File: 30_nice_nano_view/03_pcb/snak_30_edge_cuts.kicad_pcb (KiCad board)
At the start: 2 copper layers, 114 x 99 mm, 118 parts

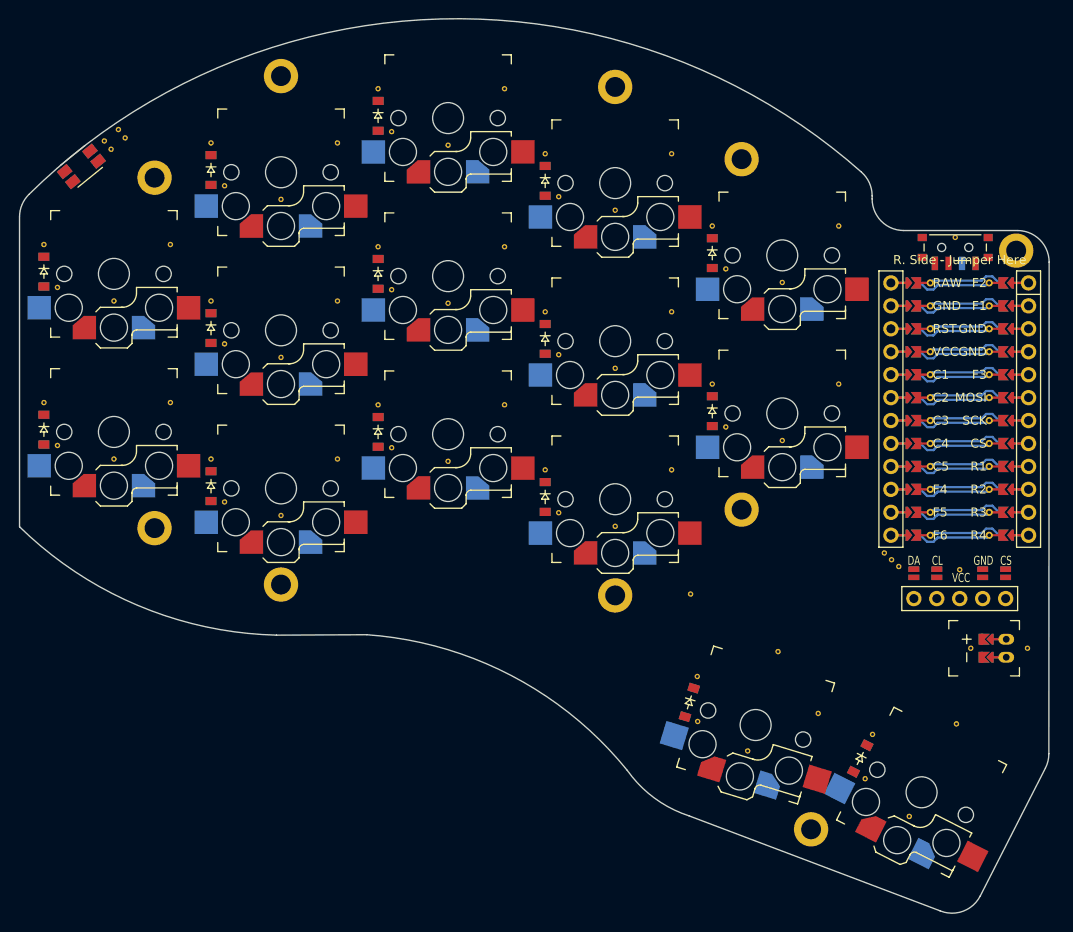
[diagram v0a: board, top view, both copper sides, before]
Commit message: update 30 key nicenano board
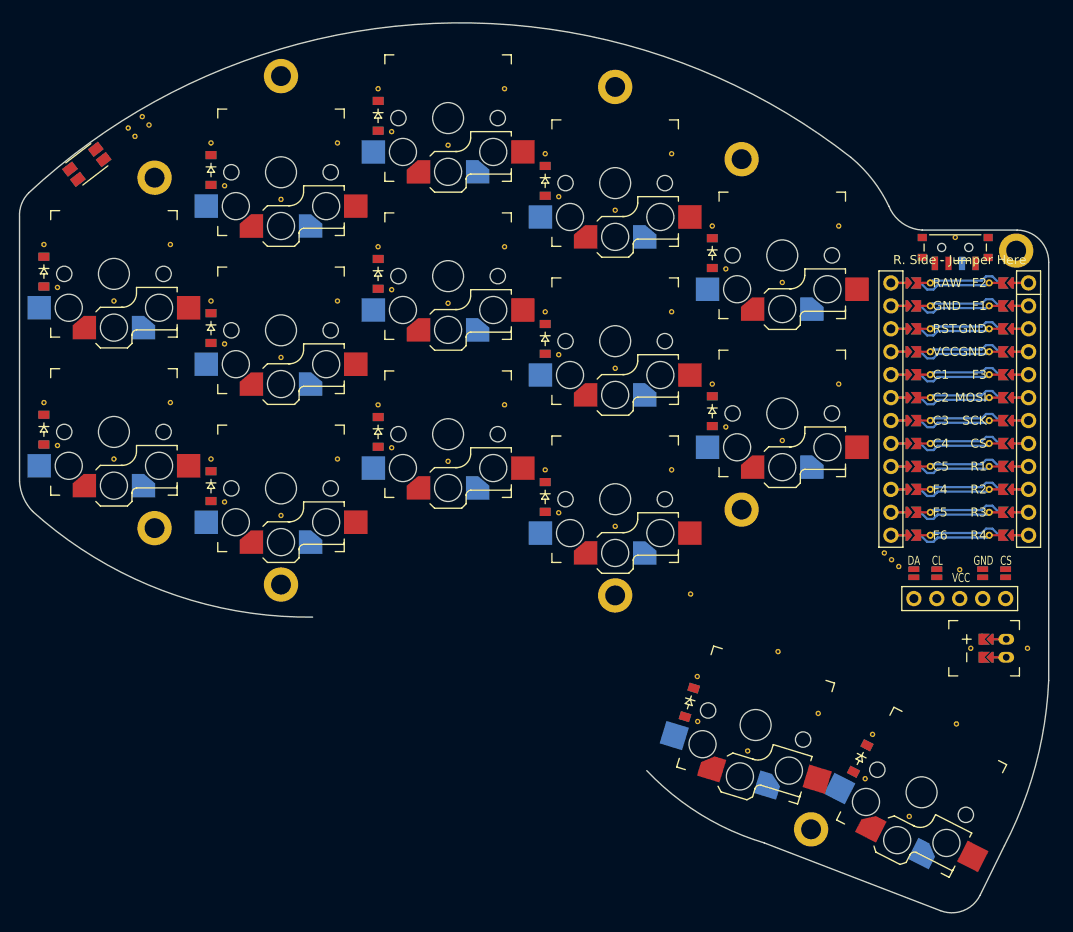
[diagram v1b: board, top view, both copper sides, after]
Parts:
- moved REF** 3.00 mm to (101.6, 48.8)
- moved REF** 3.00 mm to (102.3, 49.8)
- moved REF** 3.00 mm to (103.1, 47.6)
- moved REF** 3.00 mm to (103.9, 48.5)
- moved SW2 0.64 mm to (97.0, 52.9), turned to 127.5 degrees
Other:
- board size 114 x 99 mm -> 114 x 98.5 mm
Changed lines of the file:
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@@
   )
   (footprint "VIA-0.6mm" (layer "F.Cu")
-    (at 100.494144 49.019006 129)
+    (at 103.137109 47.589196 129)
     (attr through_hole)
     (fp_text reference "REF**" (at 0 1.4) (layer "F.SilkS") hide
@@
   )
   (footprint "VIA-0.6mm" (layer "F.Cu")
-    (at 101.243035 49.94381 129)
+    (at 103.886 48.514 129)
     (attr through_hole)
     (fp_text reference "REF**" (at 0 1.4) (layer "F.SilkS") hide
@@
   )
   (footprint "VIA-0.6mm" (layer "F.Cu")
-    (at 98.939852 50.277647 129)
+    (at 101.582817 48.847837 129)
     (attr through_hole)
     (fp_text reference "REF**" (at 0 1.4) (layer "F.SilkS") hide
@@
   )
   (footprint "sw_reset_side" (layer "F.Cu")
-    (at 96.4 53.1 129)
+    (at 97 52.87 127.5)
     (attr smd)
-    (fp_text reference "SW2" (at 0 3.5 129) (layer "F.SilkS") hide
+    (fp_text reference "SW2" (at 0 3.5 127.5) (layer "F.SilkS") hide
         (effects (font (size 1 1) (thickness 0.15)))
     )
-    (fp_text value "" (at 0 0 129) (layer "F.SilkS")
+    (fp_text value "" (at 0 0 127.5) (layer "F.SilkS")
         (effects (font (size 1.27 1.27) (thickness 0.15)))
     )
-    (fp_text user "SW2" (at 0 3.5 129) (layer "B.SilkS") hide
+    (fp_text user "SW2" (at 0 3.5 127.5) (layer "B.SilkS") hide
         (effects (font (size 1 1) (thickness 0.15)) (justify mirror))
     )
@@
     (fp_line (start 2.1 0.85) (end 2.1 -0.85)
       (stroke (width 0.1) (type solid)) (layer "F.Fab"))
-    (pad "1" smd rect (at -0.72 -1.8 219) (size 1.4 1.05) (layers "F.Cu" "F.Paste" "F.Mask")
+    (pad "1" smd rect (at -0.72 -1.8 217.5) (size 1.4 1.05) (layers "F.Cu" "F.Paste" "F.Mask")
       (net 26 "GND"))
-    (pad "1" smd rect (at -0.72 -1.8 39) (size 1.4 1.05) (layers "B.Cu" "B.Paste" "B.Mask")
+    (pad "1" smd rect (at -0.72 -1.8 37.5) (size 1.4 1.05) (layers "B.Cu" "B.Paste" "B.Mask")
       (net 26 "GND"))
-    (pad "1" smd rect (at -0.72 1.8 219) (size 1.4 1.05) (layers "F.Cu" "F.Paste" "F.Mask")
+    (pad "1" smd rect (at -0.72 1.8 217.5) (size 1.4 1.05) (layers "F.Cu" "F.Paste" "F.Mask")
       (net 26 "GND"))
-    (pad "1" smd rect (at -0.72 1.8 39) (size 1.4 1.05) (layers "B.Cu" "B.Paste" "B.Mask")
+    (pad "1" smd rect (at -0.72 1.8 37.5) (size 1.4 1.05) (layers "B.Cu" "B.Paste" "B.Mask")
       (net 26 "GND"))
-    (pad "2" smd rect (at 0.72 -1.8 219) (size 1.4 1.05) (layers "F.Cu" "F.Paste" "F.Mask")
+    (pad "2" smd rect (at 0.72 -1.8 217.5) (size 1.4 1.05) (layers "F.Cu" "F.Paste" "F.Mask")
       (net 27 "RST"))
-    (pad "2" smd rect (at 0.72 -1.8 39) (size 1.4 1.05) (layers "B.Cu" "B.Paste" "B.Mask")
+    (pad "2" smd rect (at 0.72 -1.8 37.5) (size 1.4 1.05) (layers "B.Cu" "B.Paste" "B.Mask")
       (net 27 "RST"))
-    (pad "2" smd rect (at 0.72 1.8 219) (size 1.4 1.05) (layers "F.Cu" "F.Paste" "F.Mask")
+    (pad "2" smd rect (at 0.72 1.8 217.5) (size 1.4 1.05) (layers "F.Cu" "F.Paste" "F.Mask")
       (net 27 "RST"))
-    (pad "2" smd rect (at 0.72 1.8 39) (size 1.4 1.05) (layers "B.Cu" "B.Paste" "B.Mask")
+    (pad "2" smd rect (at 0.72 1.8 37.5) (size 1.4 1.05) (layers "B.Cu" "B.Paste" "B.Mask")
       (net 27 "RST"))
   )
@@
   )
   (footprint "VIA-0.6mm" (layer "F.Cu")
-    (at 99.688743 51.20245 129)
+    (at 102.331708 49.77264 129)
     (attr through_hole)
     (fp_text reference "REF**" (at 0 1.4) (layer "F.SilkS") hide
@@
   (gr_circle (center 118.5 99.4) (end 120 99.4)
     (stroke (width 0.15) (type solid)) (fill none) (layer "Eco2.User"))
-  (gr_line (start 203.13565 119.719514) (end 195.923145 133.874853)
+  (gr_arc (start 172 128) (mid 164.97339 124.855741) (end 159 120)
     (stroke (width 0.15) (type solid)) (layer "Edge.Cuts"))
-  (gr_arc (start 187.45 60.2) (mid 184.975126 59.174874) (end 183.95 56.7)
+  (gr_line (start 198.6 128.3) (end 195.9 133.8)
     (stroke (width 0.15) (type solid)) (layer "Edge.Cuts"))
-  (gr_line (start 89.55 93) (end 89.55 58.692372)
+  (gr_arc (start 189.5 60.15) (mid 187.263797 59.364226) (end 185.8 57.5)
     (stroke (width 0.15) (type solid)) (layer "Edge.Cuts"))
-  (gr_arc (start 163.66 124.999999) (mid 159.844543 123.03625) (end 156.839956 119.972513)
+  (gr_line (start 89.55 88) (end 89.55 58.7)
     (stroke (width 0.15) (type solid)) (layer "Edge.Cuts"))
-  (gr_line (start 187.45 60.2) (end 200.048013 60.2)
+  (gr_line (start 189.5 60.15) (end 200 60.15)
     (stroke (width 0.15) (type solid)) (layer "Edge.Cuts"))
-  (gr_arc (start 89.55 58.692372) (mid 89.820936 57.342133) (end 90.591797 56.200939)
+  (gr_arc (start 89.55 58.7) (mid 89.780852 57.235609) (end 90.6 56)
     (stroke (width 0.15) (type solid)) (layer "Edge.Cuts"))
-  (gr_arc (start 203.517127 118.132533) (mid 203.42019 118.948572) (end 203.13565 119.719514)
+  (gr_arc (start 203.5 110) (mid 202.052088 119.418319) (end 198.6 128.3)
     (stroke (width 0.15) (type solid)) (layer "Edge.Cuts"))
-  (gr_line (start 183.95 56.7) (end 183.95 56.354306)
+  (gr_line (start 203.5 63.7) (end 203.5 110)
     (stroke (width 0.15) (type solid)) (layer "Edge.Cuts"))
-  (gr_line (start 203.548013 63.701986) (end 203.517127 118.132533)
+  (gr_arc (start 91 91.3) (mid 89.98406 89.777837) (end 89.55 88)
     (stroke (width 0.15) (type solid)) (layer "Edge.Cuts"))
-  (gr_arc (start 195.923145 133.874853) (mid 194.021857 135.567401) (end 191.476715 135.524198)
+  (gr_arc (start 195.9 133.8) (mid 194.031815 135.508815) (end 191.5 135.5)
     (stroke (width 0.15) (type solid)) (layer "Edge.Cuts"))
-  (gr_arc (start 200.048013 60.199999) (mid 202.523589 61.225828) (end 203.548013 63.701986)
+  (gr_arc (start 200 60.15) (mid 202.485523 61.199837) (end 203.5 63.7)
     (stroke (width 0.15) (type solid)) (layer "Edge.Cuts"))
-  (gr_arc (start 118 105) (mid 102.635557 101.701429) (end 89.55 93)
+  (gr_arc (start 181.6 52.1) (mid 183.995505 54.570163) (end 185.8 57.5)
     (stroke (width 0.15) (type solid)) (layer "Edge.Cuts"))
-  (gr_arc (start 182.771484 53.73501) (mid 183.641801 54.918199) (end 183.95 56.354306)
+  (gr_arc (start 90.6 56) (mid 135.380905 37.271116) (end 181.6 52.1)
     (stroke (width 0.15) (type solid)) (layer "Edge.Cuts"))
-  (gr_line (start 128.003322 104.952626) (end 118 105)
+  (gr_line (start 191.5 135.5) (end 172 128)
     (stroke (width 0.15) (type solid)) (layer "Edge.Cuts"))
-  (gr_arc (start 90.591797 56.200939) (mid 136.194931 36.77414) (end 182.771484 53.73501)
-    (stroke (width 0.15) (type solid)) (layer "Edge.Cuts"))
-  (gr_line (start 191.476715 135.524198) (end 163.66 125)
-    (stroke (width 0.15) (type solid)) (layer "Edge.Cuts"))
-  (gr_arc (start 128.003322 104.952626) (mid 143.983857 109.463271) (end 156.839955 119.972514)
+  (gr_arc (start 122 103) (mid 105.398912 100.067413) (end 91 91.3)
     (stroke (width 0.15) (type solid)) (layer "Edge.Cuts"))
+  (gr_arc (start 122 103) (mid 142.325339 107.527204) (end 159 120)
+    (stroke (width 0.15) (type solid)) (layer "F.Fab"))
   (segment (start 198.43 76.16) (end 196.91 76.16) (width 0.25) (layer "F.Cu") (net 1))
   (segment (start 191.11 76.51) (end 191.11 76.5) (width 0.25) (layer "B.Cu") (net 1))

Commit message: update
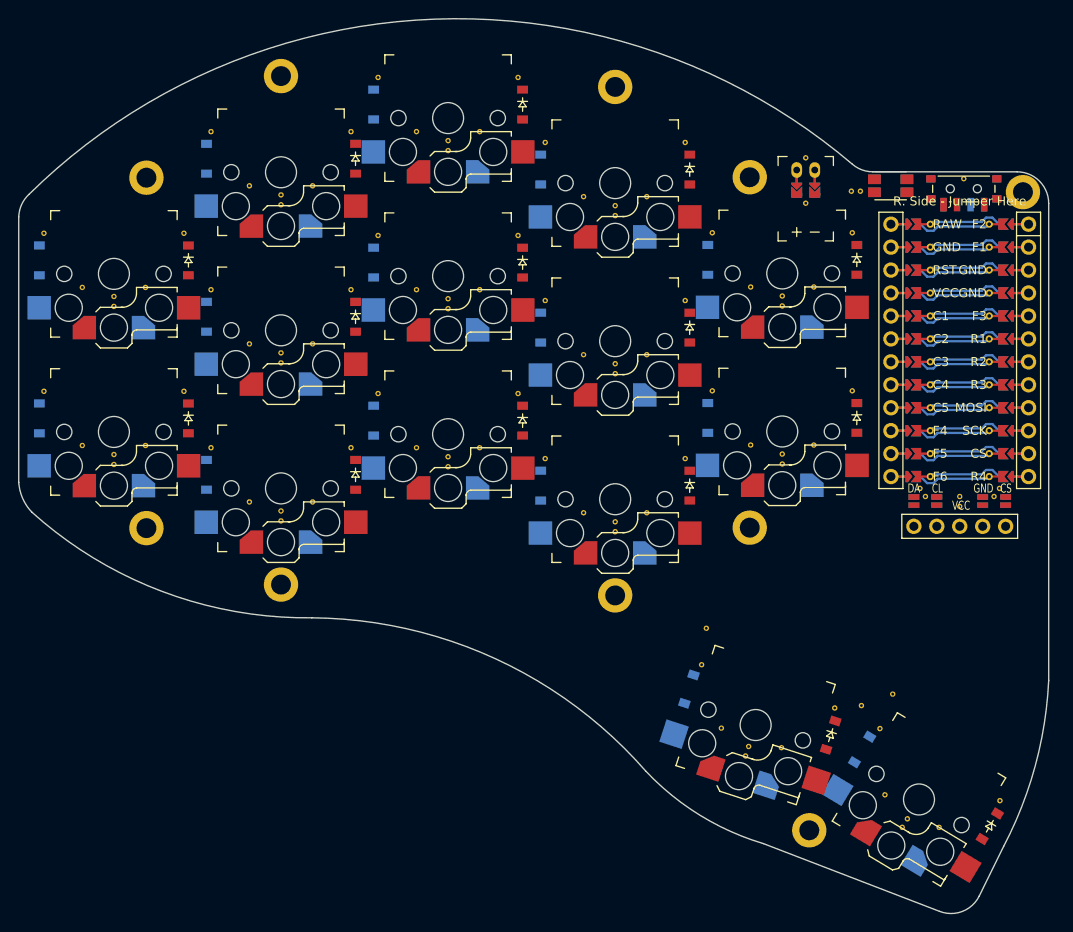
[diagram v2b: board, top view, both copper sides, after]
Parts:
- removed the REF** at (193.2, 61.0)
- removed the REF** at (161.8, 86.7)
- removed the REF** at (137.0, 85.8)
- removed the REF** at (103.1, 47.6)
- removed the REF** at (106.2, 61.8)
- removed the REF** at (106.2, 79.2)
- removed the REF** at (143.2, 79.5)
- removed the REF** at (149.2, 74.0)
- removed the REF** at (186.1, 96.7)
- removed the REF** at (118.5, 91.8)
- removed the REF** at (124.8, 50.5)
- removed the REF** at (155.5, 93.0)
- removed the REF** at (92.2, 79.2)
- removed the REF** at (184.0, 116.0)
- removed the REF** at (149.2, 56.5)
- removed the REF** at (103.9, 48.5)
- removed the REF** at (110.8, 68.0)
- removed the REF** at (174.0, 83.5)
- removed the REF** at (101.6, 48.8)
- removed the REF** at (161.8, 69.2)
- removed the REF** at (130.8, 49.2)
- removed the REF** at (100.0, 68.0)
- removed the REF** at (124.8, 85.5)
- removed the REF** at (112.2, 90.2)
- removed the REF** at (166.2, 59.7)
- removed the REF** at (118.5, 74.2)
- removed the REF** at (110.8, 85.5)
- removed the REF** at (170.2, 117.8)
- removed the REF** at (186.9, 97.4)
- removed the REF** at (155.5, 75.5)
- removed the REF** at (155.5, 58.0)
- removed the REF** at (137.0, 68.2)
- removed the REF** at (178.0, 113.7)
- removed the REF** at (124.8, 68.0)
- removed the REF** at (167.8, 64.5)
- removed the REF** at (173.5, 106.8)
- removed the REF** at (149.2, 91.5)
- removed the REF** at (130.8, 66.8)
- removed the REF** at (167.8, 82.0)
- removed the REF** at (147.8, 86.7)
- removed the REF** at (166.2, 77.2)
- removed the REF** at (164.6, 114.6)
- removed the REF** at (194.9, 106.5)
- removed the REF** at (129.2, 44.5)
- removed the REF** at (174.0, 66.0)
- removed the REF** at (118.5, 56.8)
- removed the REF** at (163.8, 100.5)
- removed the REF** at (188.1, 125.1)
- removed the REF** at (92.2, 61.8)
- removed the REF** at (183.2, 120.9)
- removed the REF** at (201.2, 106.5)
- removed the REF** at (143.2, 62.0)
- removed the REF** at (185.3, 95.9)
- removed the REF** at (147.8, 69.2)
- removed the REF** at (143.2, 44.5)
- removed the REF** at (193.3, 114.8)
- removed the REF** at (193.7, 97.8)
- removed the REF** at (110.8, 50.5)
- removed the REF** at (93.8, 84.0)
- removed the REF** at (130.8, 84.2)
- removed the REF** at (164.6, 109.6)
- removed the REF** at (137.0, 50.8)
- removed the REF** at (102.3, 49.8)
- removed the REF** at (100.0, 85.5)
- removed the REF** at (112.2, 72.8)
- removed the REF** at (180.2, 59.7)
- removed the REF** at (147.8, 51.7)
- removed the REF** at (93.8, 66.5)
- removed the REF** at (180.2, 77.2)
- removed the REF** at (129.2, 79.5)
- removed the REF** at (161.8, 51.7)
- removed the REF** at (129.2, 62.0)
- removed the REF** at (112.2, 55.2)
- added D16: , ceoloide:diode_tht_sod123, B.Cu at (91.8, 81.0)
- added D17: , ceoloide:diode_tht_sod123, B.Cu at (91.8, 63.5)
- added D18: , ceoloide:diode_tht_sod123, B.Cu at (110.2, 87.2)
- added D19: , ceoloide:diode_tht_sod123, B.Cu at (110.2, 69.8)
- added D20: , ceoloide:diode_tht_sod123, B.Cu at (110.2, 52.2)
- added D21: , ceoloide:diode_tht_sod123, B.Cu at (128.8, 81.2)
- added D22: , ceoloide:diode_tht_sod123, B.Cu at (128.8, 63.8)
- added D23: , ceoloide:diode_tht_sod123, B.Cu at (128.8, 46.2)
- added D24: , ceoloide:diode_tht_sod123, B.Cu at (147.2, 88.5)
- added D25: , ceoloide:diode_tht_sod123, B.Cu at (147.2, 71.0)
- added D26: , ceoloide:diode_tht_sod123, B.Cu at (147.2, 53.5)
- added D27: , ceoloide:diode_tht_sod123, B.Cu at (165.8, 81.0)
- added D28: , ceoloide:diode_tht_sod123, B.Cu at (165.8, 63.5)
- added D29: , ceoloide:diode_tht_sod123, B.Cu at (163.7, 111.0)
- added D30: , ceoloide:diode_tht_sod123, B.Cu at (182.8, 117.7)
- added REF**: VIA-0.6mm, VIA-0.6mm, F.Cu at (152.0, 56.5)
- added REF**: VIA-0.6mm, VIA-0.6mm, F.Cu at (107.8, 60.5)
- added REF**: VIA-0.6mm, VIA-0.6mm, F.Cu at (155.5, 57.5)
- added REF**: VIA-0.6mm, VIA-0.6mm, F.Cu at (163.2, 85.5)
- added REF**: VIA-0.6mm, VIA-0.6mm, F.Cu at (189.2, 88.8)
- added REF**: VIA-0.6mm, VIA-0.6mm, F.Cu at (122.0, 90.2)
- added REF**: VIA-0.6mm, VIA-0.6mm, F.Cu at (155.5, 92.5)
- added REF**: VIA-0.6mm, VIA-0.6mm, F.Cu at (122.0, 72.8)
- added REF**: VIA-0.6mm, VIA-0.6mm, F.Cu at (197.4, 89.7)
- added REF**: VIA-0.6mm, VIA-0.6mm, F.Cu at (144.8, 60.8)
- added REF**: VIA-0.6mm, VIA-0.6mm, F.Cu at (118.5, 73.8)
- added REF**: VIA-0.6mm, VIA-0.6mm, F.Cu at (96.5, 66.5)
- added REF**: VIA-0.6mm, VIA-0.6mm, F.Cu at (155.5, 58.5)
- added REF**: VIA-0.6mm, VIA-0.6mm, F.Cu at (118.5, 74.8)
- added REF**: VIA-0.6mm, VIA-0.6mm, F.Cu at (181.8, 60.5)
- added REF**: VIA-0.6mm, VIA-0.6mm, F.Cu at (166.2, 78.0)
- added REF**: VIA-0.6mm, VIA-0.6mm, F.Cu at (182.7, 55.8)
- added REF**: VIA-0.6mm, VIA-0.6mm, F.Cu at (167.3, 115.3)
- added REF**: VIA-0.6mm, VIA-0.6mm, F.Cu at (133.5, 66.8)
- added REF**: VIA-0.6mm, VIA-0.6mm, F.Cu at (159.0, 74.0)
- added REF**: VIA-0.6mm, VIA-0.6mm, F.Cu at (182.8, 112.8)
- added REF**: VIA-0.6mm, VIA-0.6mm, F.Cu at (137.0, 85.2)
- added REF**: VIA-0.6mm, VIA-0.6mm, F.Cu at (107.8, 78.0)
- added REF**: VIA-0.6mm, VIA-0.6mm, F.Cu at (144.8, 78.2)
- added REF**: VIA-0.6mm, VIA-0.6mm, F.Cu at (133.5, 49.2)
- added REF**: VIA-0.6mm, VIA-0.6mm, F.Cu at (179.8, 113.1)
- added REF**: VIA-0.6mm, VIA-0.6mm, F.Cu at (173.9, 117.5)
- added REF**: VIA-0.6mm, VIA-0.6mm, F.Cu at (110.8, 84.2)
- added REF**: VIA-0.6mm, VIA-0.6mm, F.Cu at (144.8, 43.2)
- added REF**: VIA-0.6mm, VIA-0.6mm, F.Cu at (103.5, 66.5)
- added REF**: VIA-0.6mm, VIA-0.6mm, F.Cu at (118.5, 91.2)
- added REF**: VIA-0.6mm, VIA-0.6mm, F.Cu at (122.0, 55.2)
- added REF**: VIA-0.6mm, VIA-0.6mm, F.Cu at (100.0, 67.5)
- added REF**: VIA-0.6mm, VIA-0.6mm, F.Cu at (163.2, 50.5)
- added REF**: VIA-0.6mm, VIA-0.6mm, F.Cu at (110.8, 66.8)
- added REF**: VIA-0.6mm, VIA-0.6mm, F.Cu at (137.0, 86.3)
- added REF**: VIA-0.6mm, VIA-0.6mm, F.Cu at (184.8, 115.3)
- added REF**: VIA-0.6mm, VIA-0.6mm, F.Cu at (129.2, 60.8)
- added REF**: VIA-0.6mm, VIA-0.6mm, F.Cu at (140.5, 84.2)
- added REF**: VIA-0.6mm, VIA-0.6mm, F.Cu at (126.2, 49.2)
- added REF**: VIA-0.6mm, VIA-0.6mm, F.Cu at (140.5, 49.2)
- added REF**: VIA-0.6mm, VIA-0.6mm, F.Cu at (126.2, 84.2)
- added REF**: VIA-0.6mm, VIA-0.6mm, F.Cu at (129.2, 43.2)
- added REF**: VIA-0.6mm, VIA-0.6mm, F.Cu at (110.8, 49.2)
- added REF**: VIA-0.6mm, VIA-0.6mm, F.Cu at (100.0, 85.0)
- added REF**: VIA-0.6mm, VIA-0.6mm, F.Cu at (155.5, 76.0)
- added REF**: VIA-0.6mm, VIA-0.6mm, F.Cu at (140.5, 66.8)
- added REF**: VIA-0.6mm, VIA-0.6mm, F.Cu at (115.0, 72.8)
- added REF**: VIA-0.6mm, VIA-0.6mm, F.Cu at (165.6, 104.2)
- added REF**: VIA-0.6mm, VIA-0.6mm, F.Cu at (137.0, 67.8)
- added REF**: VIA-0.6mm, VIA-0.6mm, F.Cu at (189.8, 89.7)
- added REF**: VIA-0.6mm, VIA-0.6mm, F.Cu at (152.0, 91.5)
- added REF**: VIA-0.6mm, VIA-0.6mm, F.Cu at (103.5, 84.0)
- added REF**: VIA-0.6mm, VIA-0.6mm, F.Cu at (155.5, 75.0)
- added REF**: VIA-0.6mm, VIA-0.6mm, F.Cu at (118.5, 56.2)
- added REF**: VIA-0.6mm, VIA-0.6mm, F.Cu at (118.5, 57.4)
- added REF**: VIA-0.6mm, VIA-0.6mm, F.Cu at (181.7, 55.8)
- added REF**: VIA-0.6mm, VIA-0.6mm, F.Cu at (198.1, 88.8)
- added REF**: VIA-0.6mm, VIA-0.6mm, F.Cu at (185.4, 122.7)
- added REF**: VIA-0.6mm, VIA-0.6mm, F.Cu at (137.0, 50.2)
- added REF**: VIA-0.6mm, VIA-0.6mm, F.Cu at (137.0, 68.8)
- added REF**: VIA-0.6mm, VIA-0.6mm, F.Cu at (159.0, 56.5)
- added REF**: VIA-0.6mm, VIA-0.6mm, F.Cu at (92.2, 78.0)
- added REF**: VIA-0.6mm, VIA-0.6mm, F.Cu at (191.4, 126.3)
- added REF**: VIA-0.6mm, VIA-0.6mm, F.Cu at (193.7, 90.8)
- added REF**: VIA-0.6mm, VIA-0.6mm, F.Cu at (115.0, 90.2)
- added REF**: VIA-0.6mm, VIA-0.6mm, F.Cu at (194.1, 54.5)
- added REF**: VIA-0.6mm, VIA-0.6mm, F.Cu at (193.7, 89.7)
- added REF**: VIA-0.6mm, VIA-0.6mm, F.Cu at (177.5, 84.0)
- added REF**: VIA-0.6mm, VIA-0.6mm, F.Cu at (170.3, 117.3)
- added REF**: VIA-0.6mm, VIA-0.6mm, F.Cu at (137.0, 51.4)
- added REF**: VIA-0.6mm, VIA-0.6mm, F.Cu at (174.0, 67.5)
- added REF**: VIA-0.6mm, VIA-0.6mm, F.Cu at (166.2, 60.5)
- added REF**: VIA-0.6mm, VIA-0.6mm, F.Cu at (176.6, 57.2)
- added REF**: VIA-0.6mm, VIA-0.6mm, F.Cu at (186.2, 111.5)
- added REF**: VIA-0.6mm, VIA-0.6mm, F.Cu at (163.2, 68.0)
- added REF**: VIA-0.6mm, VIA-0.6mm, F.Cu at (147.8, 68.0)
- added REF**: VIA-0.6mm, VIA-0.6mm, F.Cu at (133.5, 84.2)
- added REF**: VIA-0.6mm, VIA-0.6mm, F.Cu at (118.5, 92.3)
- added REF**: VIA-0.6mm, VIA-0.6mm, F.Cu at (159.0, 91.5)
- added REF**: VIA-0.6mm, VIA-0.6mm, F.Cu at (100.0, 86.1)
- added REF**: VIA-0.6mm, VIA-0.6mm, F.Cu at (174.0, 85.0)
- added REF**: VIA-0.6mm, VIA-0.6mm, F.Cu at (181.8, 78.0)
- added REF**: VIA-0.6mm, VIA-0.6mm, F.Cu at (115.0, 55.2)
- added REF**: VIA-0.6mm, VIA-0.6mm, F.Cu at (147.8, 85.5)
- added REF**: VIA-0.6mm, VIA-0.6mm, F.Cu at (187.3, 126.3)
- added REF**: VIA-0.6mm, VIA-0.6mm, F.Cu at (198.1, 123.3)
- added REF**: VIA-0.6mm, VIA-0.6mm, F.Cu at (165.1, 108.3)
- added REF**: VIA-0.6mm, VIA-0.6mm, F.Cu at (100.0, 68.6)
- added REF**: VIA-0.6mm, VIA-0.6mm, F.Cu at (96.5, 84.0)
- added REF**: VIA-0.6mm, VIA-0.6mm, F.Cu at (177.5, 66.5)
- added REF**: VIA-0.6mm, VIA-0.6mm, F.Cu at (129.2, 78.2)
- added REF**: VIA-0.6mm, VIA-0.6mm, F.Cu at (187.9, 125.3)
- added REF**: VIA-0.6mm, VIA-0.6mm, F.Cu at (174.0, 86.0)
- added REF**: VIA-0.6mm, VIA-0.6mm, F.Cu at (147.8, 50.5)
- added REF**: VIA-0.6mm, VIA-0.6mm, F.Cu at (170.5, 84.0)
- added REF**: VIA-0.6mm, VIA-0.6mm, F.Cu at (126.2, 66.8)
- added REF**: VIA-0.6mm, VIA-0.6mm, F.Cu at (170.5, 66.5)
- added REF**: VIA-0.6mm, VIA-0.6mm, F.Cu at (155.5, 93.5)
- added REF**: VIA-0.6mm, VIA-0.6mm, F.Cu at (92.2, 60.5)
- added REF**: VIA-0.6mm, VIA-0.6mm, F.Cu at (176.6, 52.1)
- added REF**: VIA-0.6mm, VIA-0.6mm, F.Cu at (152.0, 74.0)
- added REF**: VIA-0.6mm, VIA-0.6mm, F.Cu at (174.0, 68.5)
- added REF**: VIA-0.6mm, VIA-0.6mm, F.Cu at (169.9, 118.4)
- D1, D10, D11, D12, D13, D14, D15, D2, D3, D4, D5, D6, D7, D8, D9: footprint ComboDiode -> ceoloide:diode_tht_sod123
- moved SW2 89.0 mm to (186.0, 55.2), turned to 90 degrees
- moved JST1 57.4 mm to (176.6, 53.5), turned to 0 degrees
- moved D15 16.2 mm to (197.0, 126.2), turned to -121 degrees
- moved D14 16.1 mm to (179.4, 116.1), turned to -108 degrees
- moved D1 16.0 mm to (108.2, 81.0)
- moved D10 16.0 mm to (163.8, 71.0)
- moved D11 16.0 mm to (163.8, 53.5)
- moved D2 16.0 mm to (108.2, 63.5)
- moved D3 16.0 mm to (126.8, 87.2)
- moved D4 16.0 mm to (126.8, 69.8)
- moved D5 16.0 mm to (126.8, 52.2)
- moved D6 16.0 mm to (145.2, 81.2)
- moved D7 16.0 mm to (145.2, 63.8)
- moved D8 16.0 mm to (145.2, 46.2)
- moved D9 16.0 mm to (163.8, 88.5)
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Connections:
- MCU1 pad 114: R3 -> CS
- MCU1 pad 115: R2 -> SCK
- MCU1 pad 116: R1 -> MOSI
- MCU1 pad 117: CS -> R3
- MCU1 pad 118: SCK -> R2
- MCU1 pad 119: MOSI -> R1
- S3 pad 1: C1 -> C2
- S6 pad 1: C2 -> C3
- S9 pad 1: C3 -> C4
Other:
- board size 114 x 98.5 mm -> 114 x 99.1 mm
